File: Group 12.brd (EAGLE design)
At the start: 160 x 100 mm, 36 parts, among them J1 6_PIN_SERIAL_CABLEPTH, U1 328P, Y1 16MHz

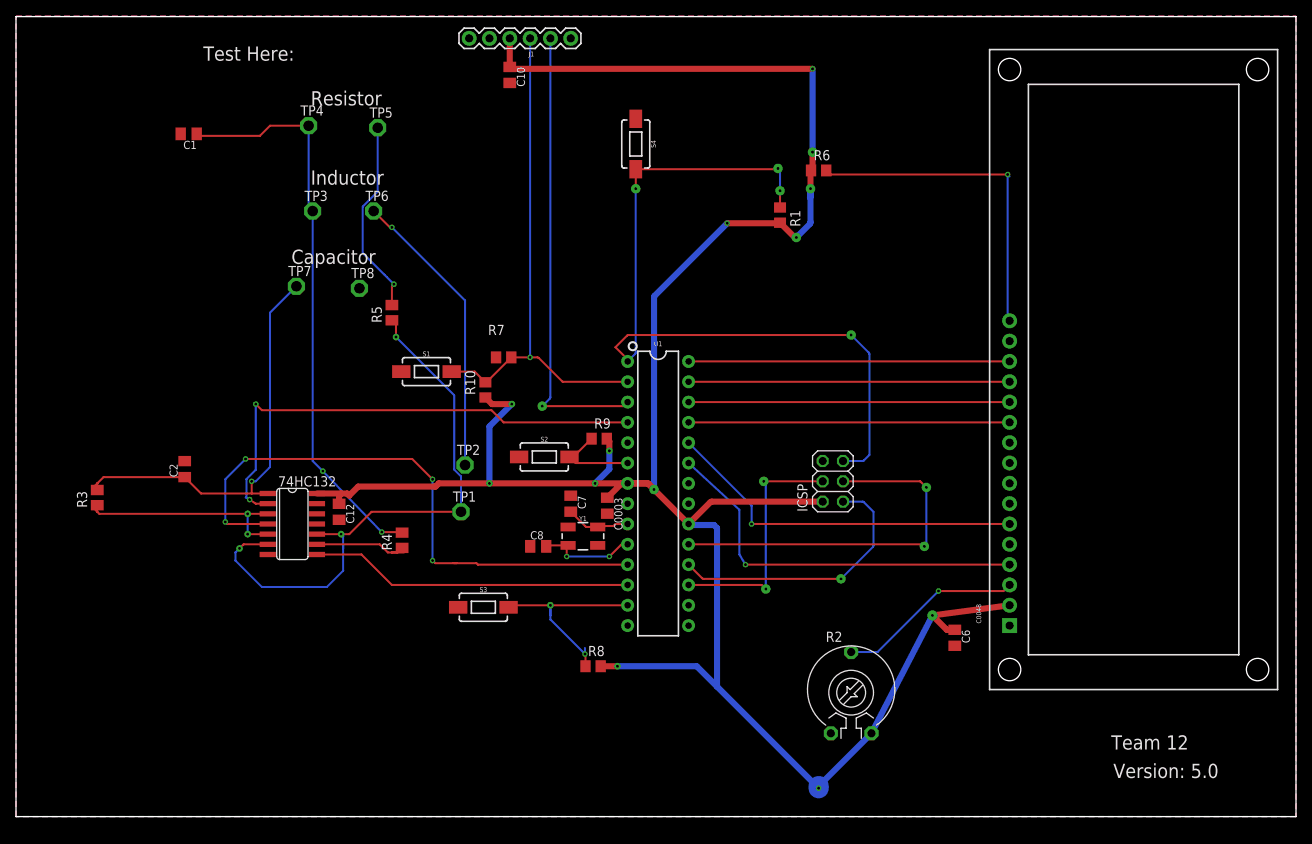
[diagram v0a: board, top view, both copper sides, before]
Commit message: final sch and brd
final sch and brd
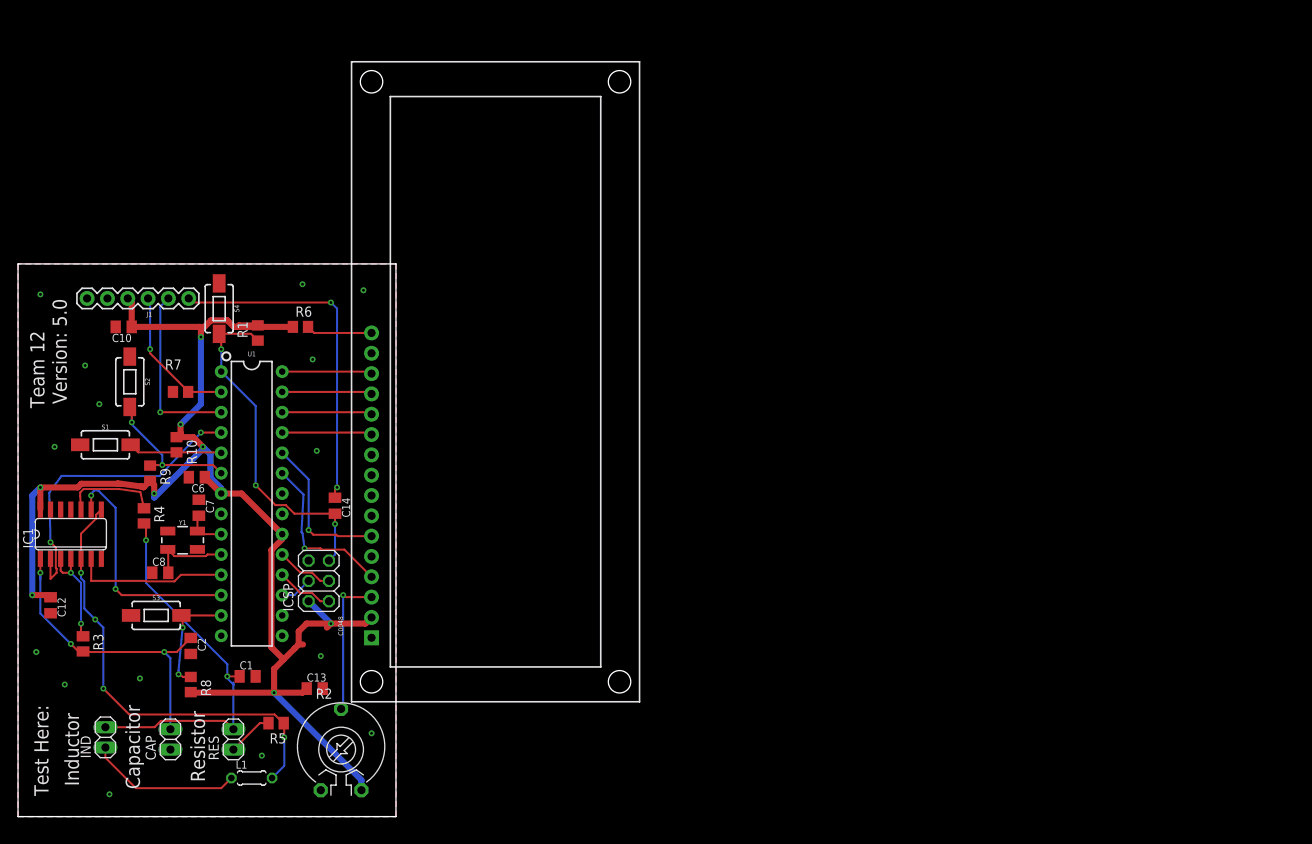
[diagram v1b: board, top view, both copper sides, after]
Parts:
- removed 74HC132: 4093D, adafruit:SO14
- removed C0003: 100n, rcl:C0805K
- removed TP1, TP2, TP3, TP4, TP5, TP6, TP7, TP8: TPPAD1-13, testpad:P1-13
- added C13: 100n, rcl:C0805K
- added C14: .1u, rcl:C0805K
- added CAP, IND, RES: (no value), pinhead:1X02
- added IC1: 74LS132D, 74xx-us:SO14
- added L1: 1m, rcl:0204/5
- R7: value 220 -> 10k
- moved C6 96.8 mm to (22.6, 42.4), turned to 180 degrees
- moved C0048 79.8 mm to (59.9, 54.4)
- moved C1 68.2 mm to (29.0, 17.5), turned to 0 degrees
- moved R6 67.7 mm to (35.6, 61.2)
- moved R1 66.9 mm to (30.2, 60.5), turned to 90 degrees
- moved ICSP 65.5 mm to (37.8, 29.5)
- moved R2 64.1 mm to (40.6, 8.38)
- moved J1 57.8 mm to (21.6, 64.8)
- moved C10 57.6 mm to (13.5, 61.2), turned to 180 degrees
- moved R9 56.3 mm to (16.8, 42.9), turned to 270 degrees
- moved S4 56.0 mm to (25.4, 63.5)
- moved R5 53.3 mm to (32.5, 11.7), turned to 180 degrees
- moved S2 52.7 mm to (14.2, 54.4), turned to 270 degrees
- moved U1 50.8 mm to (29.5, 39.1)
- moved R8 50.3 mm to (21.8, 16.5), turned to 270 degrees
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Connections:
- new net MODE: R10.2, S1.2, U1.5
- new net N$7: C14.1, J1.DTR
- net 5V: now also C13.1, IC1.14; no longer 74HC132.14, C0003.1
- net GND: now also C13.2, CAP.1, IC1.12, IC1.13, IC1.7; no longer 74HC132.11, 74HC132.12, 74HC132.13, 74HC132.7, C0003.2, TP8.TP
- net N$1: now also C2.1, CAP.2, IC1.1, R3.2; no longer 74HC132.9, R4.1
- net N$10: now also IC1.5, IC1.8, L1.2; no longer 74HC132.10, 74HC132.6, TP1.TP
- net N$14: now also IND.1, L1.1; no longer TP2.TP, TP6.TP
- net N$16: now also IND.2, RES.2; no longer TP3.TP, TP4.TP
- net N$17: now also RES.1; no longer TP5.TP
- net N$2: now also IC1.10, R4.1; no longer 74HC132.1, C2.1, R3.2, TP7.TP
- net N$5: now also IC1.3, IC1.4; no longer 74HC132.3, 74HC132.5
- net PD0: no longer R10.2, S1.2
- net PD2: now also IC1.2; no longer 74HC132.2
- net PD5: now also IC1.6; no longer 74HC132.4
- net PD6: now also IC1.9; no longer 74HC132.8
- net RESET: now also C14.2
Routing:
- net 5V: track 319.0 -> 182.4 mm, vias 13 -> 8
- net RESET: track 99.2 -> 43.5 mm, vias 4 -> 3
- net PD5: track 74.0 -> 19.4 mm, vias 4 -> 0
- net PD0: track 65.0 -> 17.9 mm
- net N$7: track 0.00 -> 42.8 mm, vias 0 -> 2
- net N$2: track 52.5 -> 12.0 mm, vias 1 -> 0
- net SCK: track 47.7 -> 7.21 mm, vias 2 -> 0
- net N$3: track 57.2 -> 22.3 mm
- net N$22: track 41.6 -> 8.25 mm, vias 1 -> 0
- net PC4: track 41.4 -> 11.3 mm
- net PC3: track 40.1 -> 11.3 mm
- net PC2: track 40.1 -> 11.3 mm
- net PC5: track 40.1 -> 11.4 mm
- net PC0: track 48.7 -> 20.4 mm
- net MISO: track 34.1 -> 7.21 mm, vias 1 -> 0
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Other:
- board size 160 x 100 mm -> 47.2 x 69.1 mm
